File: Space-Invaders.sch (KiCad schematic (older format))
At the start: 73 parts, among them Q1 BS170, Q2 BS170, Q3 BS170, Q4 BS170, U1 LM556, U2 LM3900, U3 4070, U4 CD4006, U5 LM358, U6 LM386

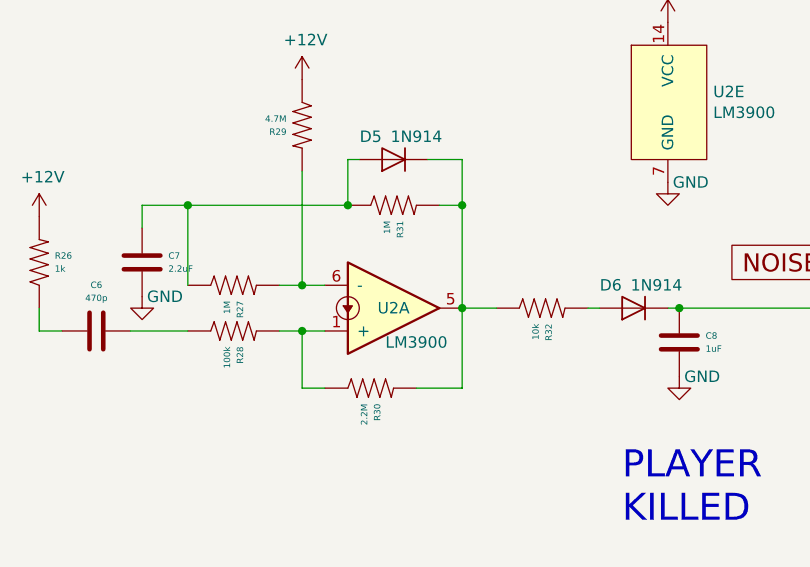
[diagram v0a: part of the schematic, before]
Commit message: gg
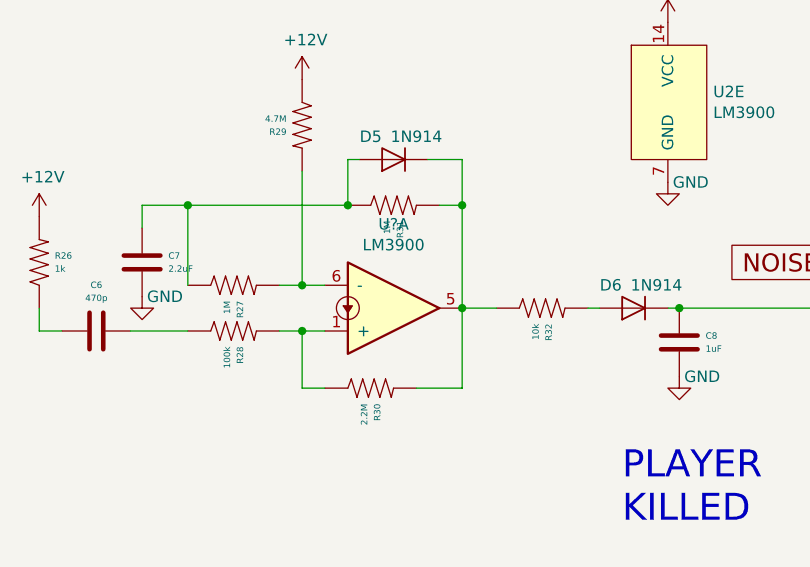
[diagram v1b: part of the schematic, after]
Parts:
- removed unit 1 of U2
- added U?: LM3900, symbol Xenir:LM3900
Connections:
- net at R28.2, R30.1: now also U?.1 (+)
- net at D5.1 (K), R30.2, R31.2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: now also U?.5
- net at R27.2, R29.2: now also U?.6 (-)
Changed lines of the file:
@@
-$Comp
-L Xenir:LM3900 U2
-U 1 1 634082C5
-P 8250 5000
-F 0 "U2" H 8250 5000 50  0000 C CNN
-F 1 "LM3900" H 8350 4850 50  0000 C CNN
-F 2 "" H 8130 5050 50  0001 C CNN
-F 3 "" H 8130 5050 50  0001 C CNN
-	1    8250 5000
-	1    0    0    -1
-$EndComp
 $Comp
 L Xenir:LM3900 U2
@@
 Text Notes 3800 2600 0    118  ~ 0
 FET DRIVER CIRCUIT\n(not original)
+$Comp
+L Xenir:LM3900 U?
+U 1 1 6341538E
+P 8250 5000
+F 0 "U?" H 8250 5367 50  0000 C CNN
+F 1 "LM3900" H 8250 5276 50  0000 C CNN
+F 2 "" H 8130 5050 50  0001 C CNN
+F 3 "" H 8130 5050 50  0001 C CNN
+	1    8250 5000
+	1    0    0    -1
+$EndComp
 $EndSCHEMATC
